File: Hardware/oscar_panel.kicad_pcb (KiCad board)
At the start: 2 copper layers, 71 x 128.5 mm, 11 parts

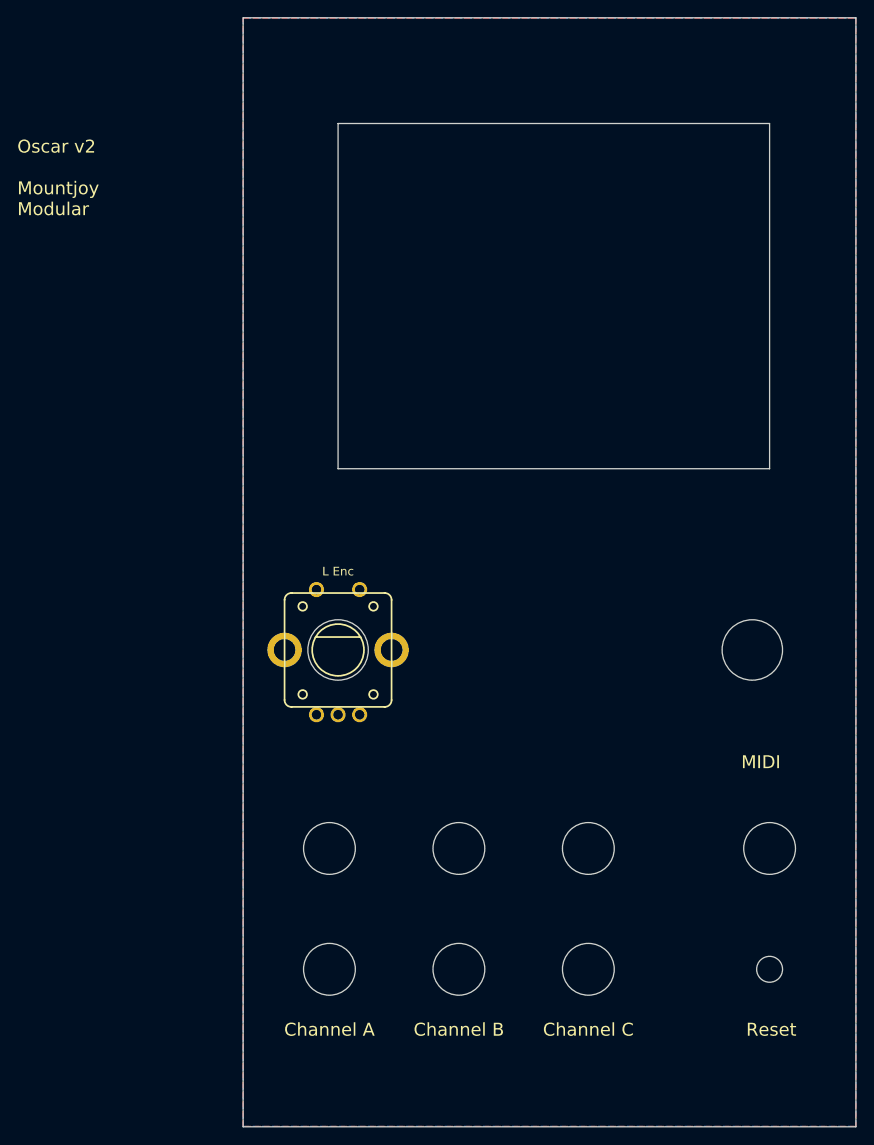
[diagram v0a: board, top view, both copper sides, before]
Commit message: Updates to panel PCB
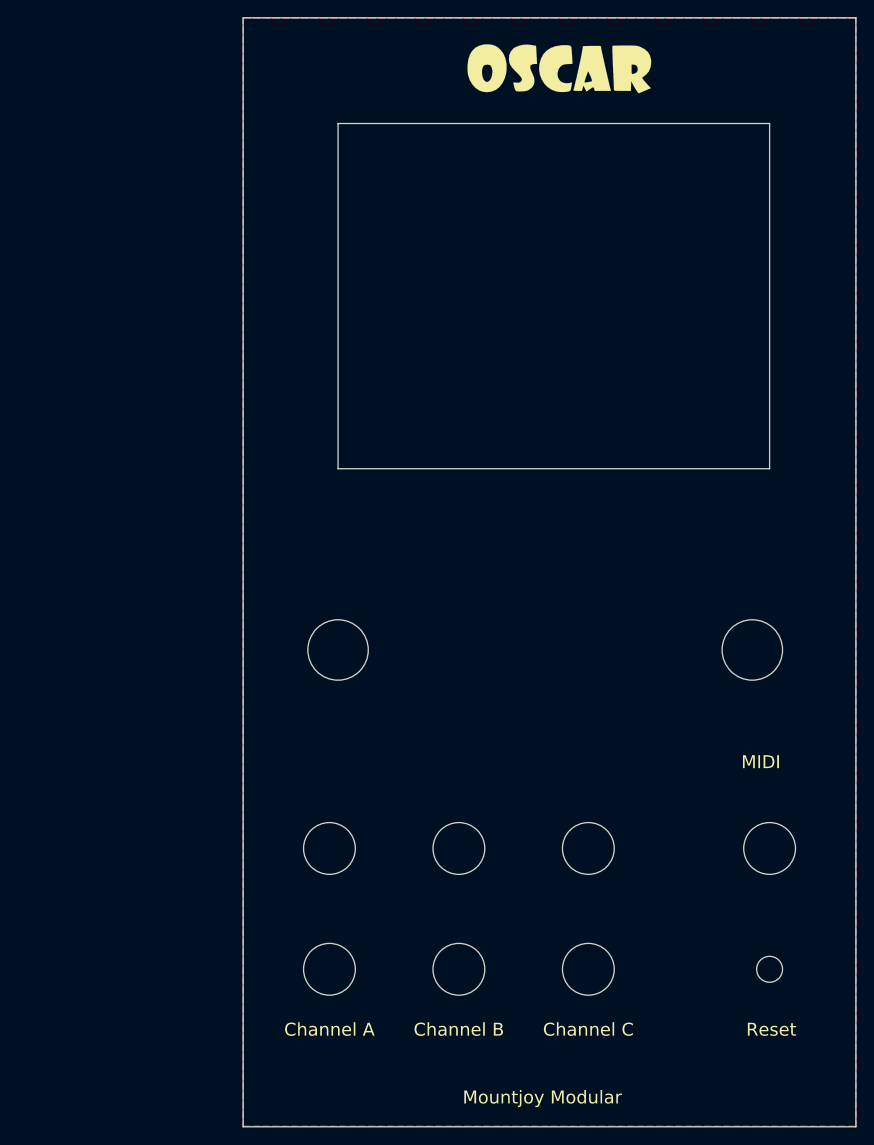
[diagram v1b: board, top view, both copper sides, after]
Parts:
- removed L Enc: Left_Encoder, Custom_Footprints:Encoder
- added G***: LOGO, oscar_logo:oscar_logo, F.Cu at (162.6, 46.9)
- added Ref**: Oval_Mounting_Hole, Custom_Footprints:Oval_Mounting_Hole, F.Cu at (188.5, 166.2)
- added Ref**: Oval_Mounting_Hole, Custom_Footprints:Oval_Mounting_Hole, F.Cu at (132.5, 166.2)
- added Ref**: Oval_Mounting_Hole, Custom_Footprints:Oval_Mounting_Hole, F.Cu at (188.5, 43.8)
- added Ref**: Oval_Mounting_Hole, Custom_Footprints:Oval_Mounting_Hole, F.Cu at (132.5, 43.8)
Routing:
- added copper zone on B.Cu, net (none)
- added copper zone on F.Cu, net (none)
- removed copper zone on B.Cu, net GND
- removed copper zone on F.Cu, net GND
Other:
- board text added: "Mountjoy Modular"
- board text removed: "Oscar v2 Mountjoy Modular"

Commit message: updated codebase
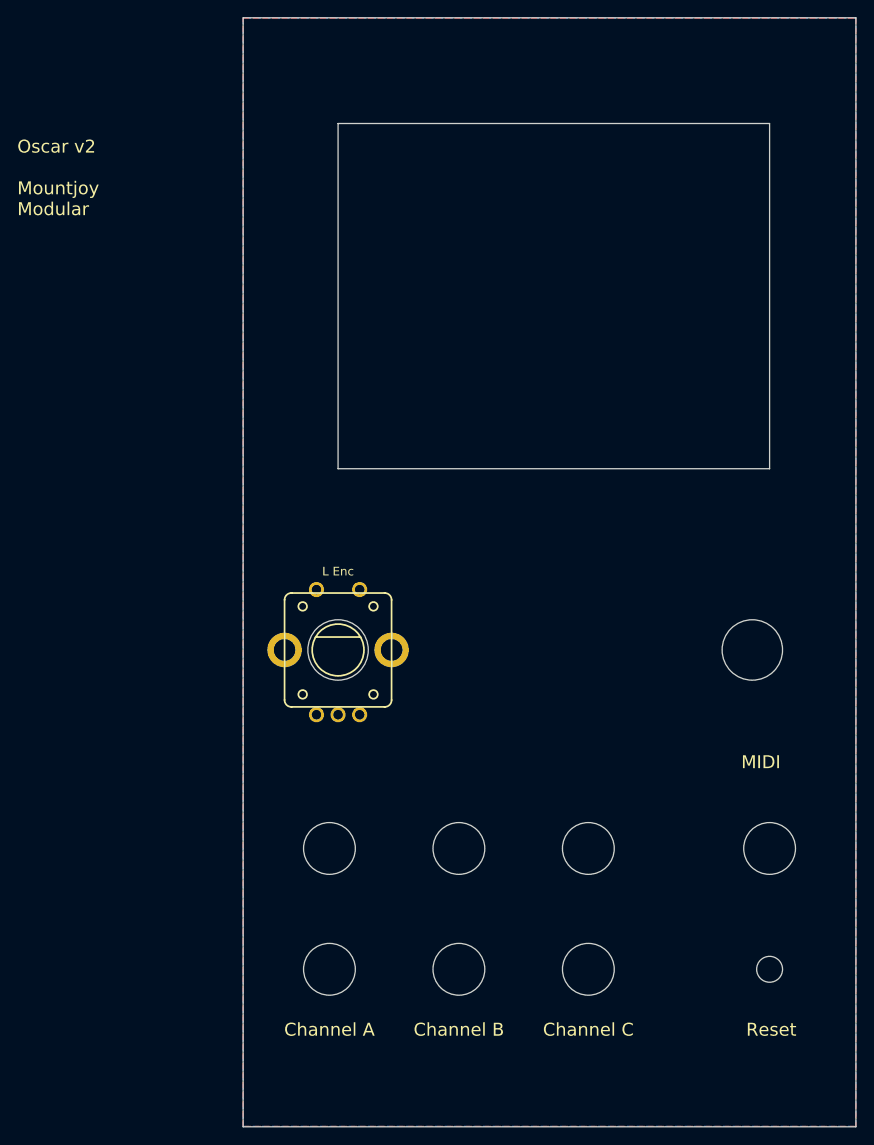
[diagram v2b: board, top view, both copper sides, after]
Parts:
- removed G***: LOGO, oscar_logo:oscar_logo
- removed the Ref** at (188.5, 166.2)
- removed the Ref** at (132.5, 166.2)
- removed the Ref** at (188.5, 43.8)
- removed the Ref** at (132.5, 43.8)
- added L Enc: Left_Encoder, Custom_Footprints:Encoder, F.Cu at (136.0, 114.0)
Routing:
- added copper zone on B.Cu, net GND
- added copper zone on F.Cu, net GND
- removed copper zone on B.Cu, net (none)
- removed copper zone on F.Cu, net (none)
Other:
- board text added: "Oscar v2 Mountjoy Modular"
- board text removed: "Mountjoy Modular"
